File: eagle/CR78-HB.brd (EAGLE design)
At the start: 100 x 80 mm, 34 parts, among them Q1 2N3904, Q2 2N3904, Q3 2N3904, X1 22-23-2021

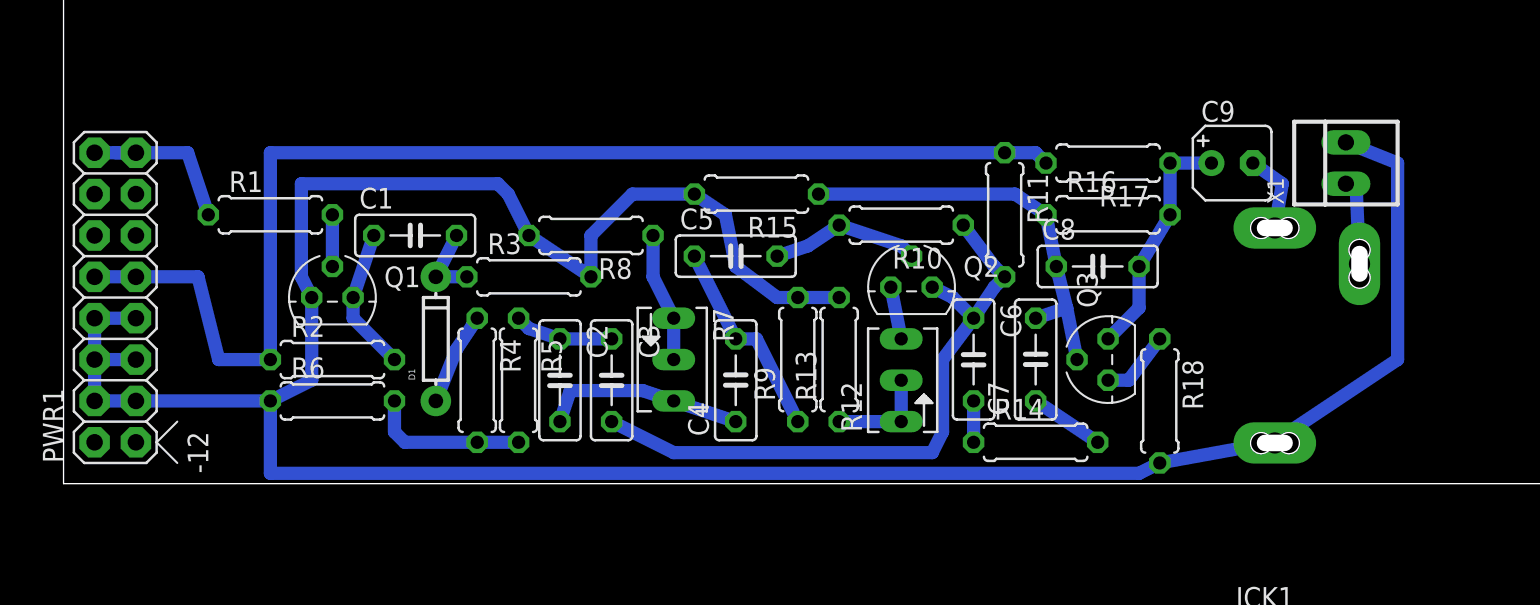
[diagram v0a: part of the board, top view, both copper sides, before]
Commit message: cutout
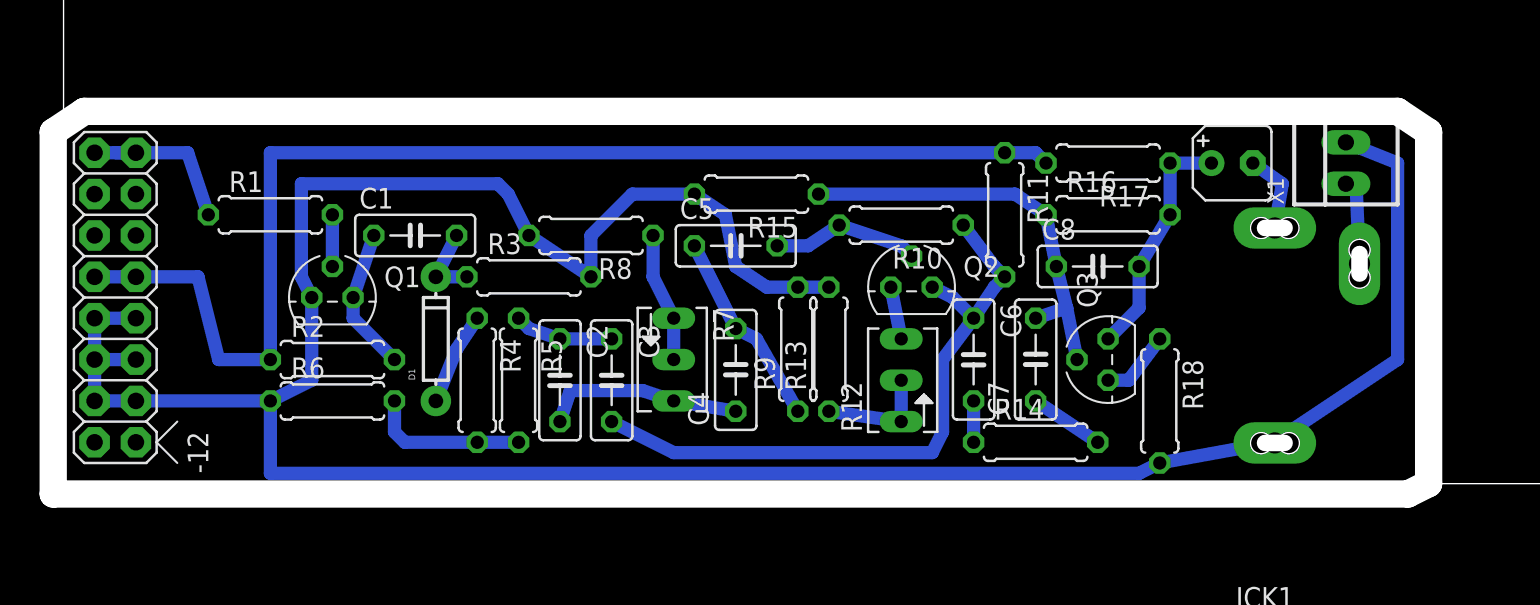
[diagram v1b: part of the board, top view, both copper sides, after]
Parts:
- moved R13 0.90 mm to (47.0, 8.26)
- moved C4 0.64 mm to (41.3, 6.99)
- moved R9 0.64 mm to (45.1, 8.26)
- moved C5 0.63 mm to (41.3, 14.6)
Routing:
- net GND: track 169.8 -> 168.9 mm
- net N$8: track 6.35 -> 7.03 mm
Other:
- board size 100 x 80 mm -> 100.6 x 80.6 mm
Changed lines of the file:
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@@
 <layer number="44" name="Drills" color="7" fill="1" visible="no" active="yes"/>
 <layer number="45" name="Holes" color="7" fill="1" visible="no" active="yes"/>
-<layer number="46" name="Milling" color="3" fill="1" visible="no" active="yes"/>
+<layer number="46" name="Milling" color="3" fill="1" visible="yes" active="yes"/>
 <layer number="47" name="Measures" color="7" fill="1" visible="no" active="yes"/>
 <layer number="48" name="Document" color="7" fill="1" visible="yes" active="yes"/>
@@
 <wire x1="100" y1="80" x2="0" y2="80" width="0" layer="20"/>
 <wire x1="0" y1="80" x2="0" y2="0" width="0" layer="20"/>
+<wire x1="-0.635" y1="-0.635" x2="-0.635" y2="21.59" width="1.6764" layer="46"/>
+<wire x1="-0.635" y1="21.59" x2="1.27" y2="22.86" width="1.6764" layer="46"/>
+<wire x1="1.27" y1="22.86" x2="81.915" y2="22.86" width="1.6764" layer="46"/>
+<wire x1="81.915" y1="22.86" x2="83.82" y2="21.59" width="1.6764" layer="46"/>
+<wire x1="83.82" y1="21.59" x2="83.82" y2="0" width="1.6764" layer="46"/>
+<wire x1="83.82" y1="0" x2="82.55" y2="-0.635" width="1.6764" layer="46"/>
+<wire x1="82.55" y1="-0.635" x2="-0.635" y2="-0.635" width="1.6764" layer="46"/>
 </plain>
 <attributes>
@@
 <element name="C2" library="rcl" package="C050-025X075" value="8n2" x="30.48" y="6.35" rot="R270"/>
 <element name="C3" library="rcl" package="C050-025X075" value="8n2" x="33.655" y="6.35" rot="R270"/>
-<element name="C4" library="rcl" package="C050-025X075" value="6n8" x="41.275" y="6.35" rot="R90"/>
-<element name="C5" library="rcl" package="C050-025X075" value="6n8" x="41.275" y="13.97"/>
+<element name="C4" library="rcl" package="C050-025X075" value="6n8" x="41.275" y="6.985" rot="R90"/>
+<element name="C5" library="rcl" package="C050-025X075" value="6n8" x="41.275" y="14.605"/>
 <element name="C6" library="rcl" package="C050-025X075" value="2n2" x="55.88" y="7.62" rot="R270"/>
 <element name="C7" library="rcl" package="C050-025X075" value="473" x="59.69" y="7.62" rot="R90"/>
@@
 <element name="R5" library="rcl" package="0207/7" value="15k" x="27.94" y="6.35" rot="R270"/>
 <element name="R8" library="rcl" package="0207/7" value="10k" x="32.385" y="15.24" rot="R180"/>
-<element name="R9" library="rcl" package="0207/7" value="15k" x="45.085" y="7.62" rot="R90"/>
-<element name="R13" library="rcl" package="0207/7" value="100R" x="47.625" y="7.62" rot="R90"/>
+<element name="R9" library="rcl" package="0207/7" value="15k" x="45.085" y="8.255" rot="R90"/>
+<element name="R13" library="rcl" package="0207/7" value="100R" x="46.99" y="8.255" rot="R90"/>
 <element name="R10" library="rcl" package="0207/7" value="1M5" x="51.435" y="15.875" rot="R180"/>
 <element name="R11" library="rcl" package="0207/7" value="10k" x="57.785" y="16.51" rot="R270"/>
@@
 <wire x1="1.905" y1="7.62" x2="1.905" y2="10.16" width="0.8128" layer="16"/>
 <wire x1="4.445" y1="5.08" x2="12.7" y2="5.08" width="0.8128" layer="16"/>
-<wire x1="47.625" y1="11.43" x2="45.085" y2="11.43" width="0.8128" layer="16"/>
+<wire x1="46.99" y1="12.065" x2="45.085" y2="12.065" width="0.8128" layer="16"/>
 <wire x1="14.605" y1="12.7" x2="15.24" y2="11.43" width="0.8128" layer="16"/>
 <wire x1="14.605" y1="18.415" x2="14.605" y2="12.7" width="0.8128" layer="16"/>
@@
 <wire x1="12.7" y1="0.635" x2="66.04" y2="0.635" width="0.8128" layer="16"/>
 <wire x1="12.7" y1="5.08" x2="12.7" y2="0.635" width="0.8128" layer="16"/>
-<wire x1="41.275" y1="13.335" x2="43.815" y2="11.43" width="0.8128" layer="16"/>
-<wire x1="43.815" y1="11.43" x2="45.085" y2="11.43" width="0.8128" layer="16"/>
+<wire x1="41.275" y1="13.335" x2="43.18" y2="12.065" width="0.8128" layer="16"/>
+<wire x1="43.18" y1="12.065" x2="45.085" y2="12.065" width="0.8128" layer="16"/>
 <wire x1="28.575" y1="15.24" x2="27.305" y2="17.78" width="0.8128" layer="16"/>
 <wire x1="27.305" y1="17.78" x2="26.67" y2="18.415" width="0.8128" layer="16"/>
@@
 <wire x1="35.56" y1="5.715" x2="31.115" y2="5.715" width="0.8128" layer="16"/>
 <wire x1="37.465" y1="5.08" x2="35.56" y2="5.715" width="0.8128" layer="16"/>
-<wire x1="37.465" y1="5.08" x2="41.275" y2="3.81" width="0.8128" layer="16"/>
+<wire x1="37.465" y1="5.08" x2="41.275" y2="4.445" width="0.8128" layer="16"/>
 </signal>
 <signal name="N$7">
@@
 <wire x1="47.625" y1="15.875" x2="51.435" y2="14.605" width="0.8128" layer="16"/>
 <wire x1="51.435" y1="14.605" x2="52.07" y2="13.97" width="0.8128" layer="16"/>
-<wire x1="43.815" y1="13.97" x2="45.72" y2="14.605" width="0.8128" layer="16"/>
+<wire x1="43.815" y1="14.605" x2="45.72" y2="14.605" width="0.8128" layer="16"/>
 <wire x1="45.72" y1="14.605" x2="47.625" y2="15.875" width="0.8128" layer="16"/>
 </signal>
@@
 <contactref element="R13" pad="1"/>
 <contactref element="R12" pad="S"/>
-<wire x1="51.435" y1="3.81" x2="47.625" y2="3.81" width="0.8128" layer="16"/>
+<wire x1="51.435" y1="3.81" x2="46.99" y2="4.445" width="0.8128" layer="16"/>
 <wire x1="51.435" y1="3.81" x2="51.435" y2="6.35" width="0.8128" layer="16"/>
 </signal>
@@
 <contactref element="C4" pad="2"/>
 <contactref element="R9" pad="1"/>
-<wire x1="38.735" y1="13.97" x2="41.275" y2="8.89" width="0.8128" layer="16"/>
-<wire x1="41.275" y1="8.89" x2="42.545" y2="8.89" width="0.8128" layer="16"/>
-<wire x1="42.545" y1="8.89" x2="45.085" y2="3.81" width="0.8128" layer="16"/>
+<wire x1="38.735" y1="14.605" x2="41.275" y2="9.525" width="0.8128" layer="16"/>
+<wire x1="41.275" y1="9.525" x2="42.545" y2="8.89" width="0.8128" layer="16"/>
+<wire x1="42.545" y1="8.89" x2="45.085" y2="4.445" width="0.8128" layer="16"/>
 </signal>
 <signal name="N$11">

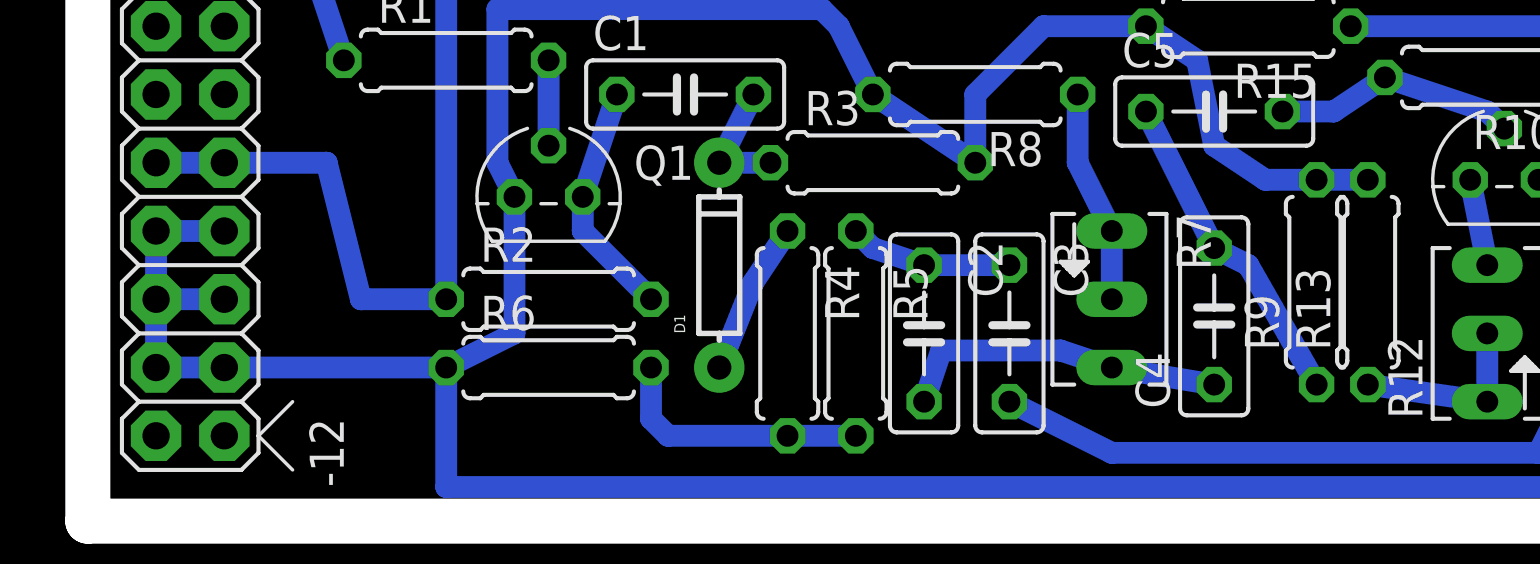
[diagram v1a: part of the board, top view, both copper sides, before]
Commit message: gcode
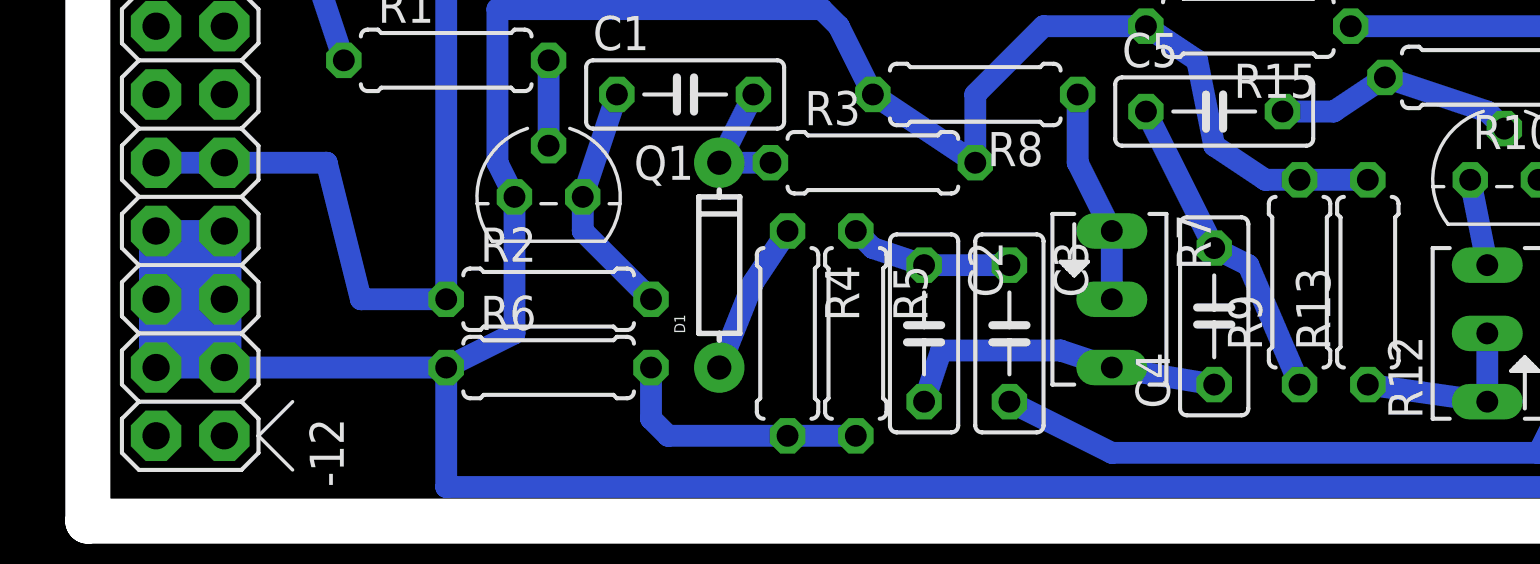
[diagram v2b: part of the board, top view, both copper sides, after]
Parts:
- moved R9 0.63 mm to (44.5, 8.26)
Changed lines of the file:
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@@
 <?xml version="1.0" encoding="utf-8"?>
 <!DOCTYPE eagle SYSTEM "eagle.dtd">
-<eagle version="7.2.0">
+<eagle version="7.1.0">
 <drawing>
 <settings>
@@
 <wire x1="83.82" y1="0" x2="82.55" y2="-0.635" width="1.6764" layer="46"/>
 <wire x1="82.55" y1="-0.635" x2="-0.635" y2="-0.635" width="1.6764" layer="46"/>
+<rectangle x1="1.27" y1="5.08" x2="5.08" y2="10.16" layer="16"/>
 </plain>
 <attributes>
@@
 <element name="R5" library="rcl" package="0207/7" value="15k" x="27.94" y="6.35" rot="R270"/>
 <element name="R8" library="rcl" package="0207/7" value="10k" x="32.385" y="15.24" rot="R180"/>
-<element name="R9" library="rcl" package="0207/7" value="15k" x="45.085" y="8.255" rot="R90"/>
+<element name="R9" library="rcl" package="0207/7" value="15k" x="44.45" y="8.255" rot="R90"/>
 <element name="R13" library="rcl" package="0207/7" value="100R" x="46.99" y="8.255" rot="R90"/>
 <element name="R10" library="rcl" package="0207/7" value="1M5" x="51.435" y="15.875" rot="R180"/>
@@
 <wire x1="1.905" y1="7.62" x2="1.905" y2="10.16" width="0.8128" layer="16"/>
 <wire x1="4.445" y1="5.08" x2="12.7" y2="5.08" width="0.8128" layer="16"/>
-<wire x1="46.99" y1="12.065" x2="45.085" y2="12.065" width="0.8128" layer="16"/>
+<wire x1="46.99" y1="12.065" x2="44.45" y2="12.065" width="0.8128" layer="16"/>
 <wire x1="14.605" y1="12.7" x2="15.24" y2="11.43" width="0.8128" layer="16"/>
 <wire x1="14.605" y1="18.415" x2="14.605" y2="12.7" width="0.8128" layer="16"/>
@@
 <wire x1="12.7" y1="5.08" x2="12.7" y2="0.635" width="0.8128" layer="16"/>
 <wire x1="41.275" y1="13.335" x2="43.18" y2="12.065" width="0.8128" layer="16"/>
-<wire x1="43.18" y1="12.065" x2="45.085" y2="12.065" width="0.8128" layer="16"/>
+<wire x1="43.18" y1="12.065" x2="44.45" y2="12.065" width="0.8128" layer="16"/>
 <wire x1="28.575" y1="15.24" x2="27.305" y2="17.78" width="0.8128" layer="16"/>
 <wire x1="27.305" y1="17.78" x2="26.67" y2="18.415" width="0.8128" layer="16"/>
@@
 <wire x1="38.735" y1="14.605" x2="41.275" y2="9.525" width="0.8128" layer="16"/>
 <wire x1="41.275" y1="9.525" x2="42.545" y2="8.89" width="0.8128" layer="16"/>
-<wire x1="42.545" y1="8.89" x2="45.085" y2="4.445" width="0.8128" layer="16"/>
+<wire x1="42.545" y1="8.89" x2="44.45" y2="4.445" width="0.8128" layer="16"/>
 </signal>
 <signal name="N$11">

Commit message: lb
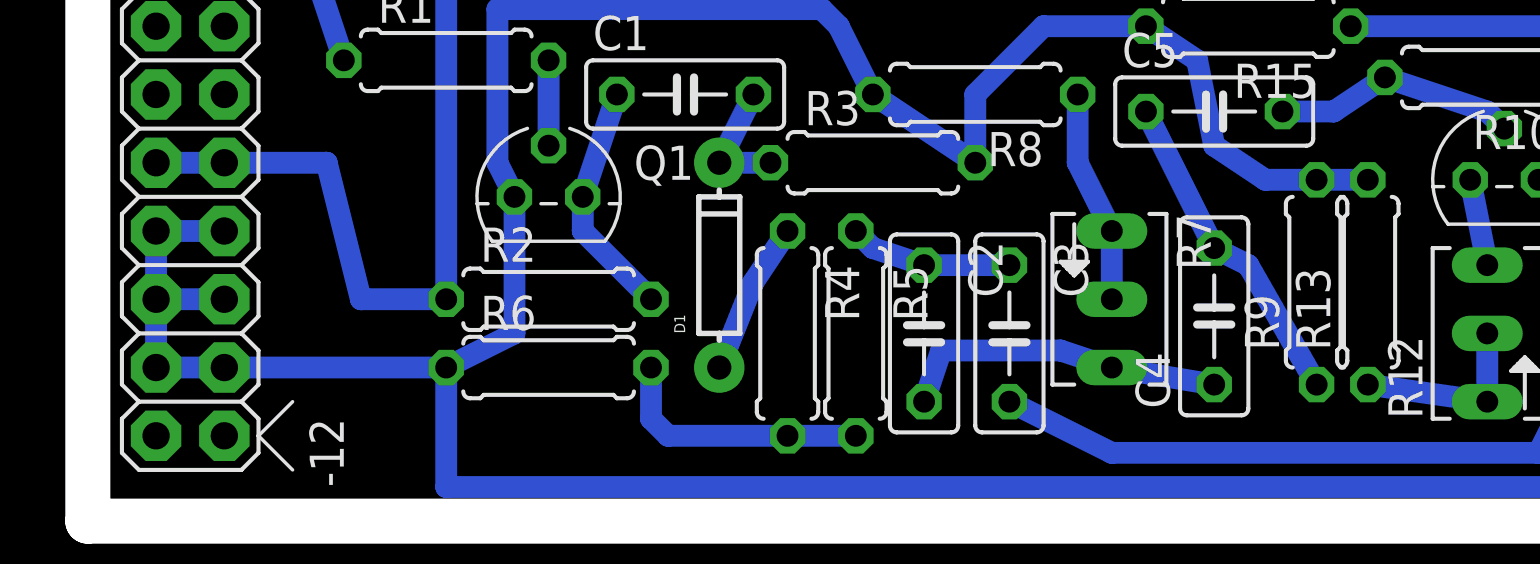
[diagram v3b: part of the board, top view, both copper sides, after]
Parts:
- C2: value 8n2 -> 12n
- C3: value 8n2 -> 18n
- C4: value 6n8 -> 12n
- C5: value 6n8 -> 10n
- C6: value 2n2 -> 8n2
- R14: value 1M5 -> 680k
- moved R9 0.63 mm to (45.1, 8.26)
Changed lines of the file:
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@@
 <?xml version="1.0" encoding="utf-8"?>
 <!DOCTYPE eagle SYSTEM "eagle.dtd">
-<eagle version="7.1.0">
+<eagle version="7.2.0">
 <drawing>
 <settings>
@@
 <wire x1="83.82" y1="0" x2="82.55" y2="-0.635" width="1.6764" layer="46"/>
 <wire x1="82.55" y1="-0.635" x2="-0.635" y2="-0.635" width="1.6764" layer="46"/>
-<rectangle x1="1.27" y1="5.08" x2="5.08" y2="10.16" layer="16"/>
 </plain>
 <attributes>
@@
 <elements>
 <element name="C1" library="rcl" package="C050-025X075" value="27n" x="21.59" y="15.24"/>
-<element name="C2" library="rcl" package="C050-025X075" value="8n2" x="30.48" y="6.35" rot="R270"/>
-<element name="C3" library="rcl" package="C050-025X075" value="8n2" x="33.655" y="6.35" rot="R270"/>
-<element name="C4" library="rcl" package="C050-025X075" value="6n8" x="41.275" y="6.985" rot="R90"/>
-<element name="C5" library="rcl" package="C050-025X075" value="6n8" x="41.275" y="14.605"/>
-<element name="C6" library="rcl" package="C050-025X075" value="2n2" x="55.88" y="7.62" rot="R270"/>
+<element name="C2" library="rcl" package="C050-025X075" value="12n" x="30.48" y="6.35" rot="R270"/>
+<element name="C3" library="rcl" package="C050-025X075" value="18n" x="33.655" y="6.35" rot="R270"/>
+<element name="C4" library="rcl" package="C050-025X075" value="12n" x="41.275" y="6.985" rot="R90"/>
+<element name="C5" library="rcl" package="C050-025X075" value="10n" x="41.275" y="14.605"/>
+<element name="C6" library="rcl" package="C050-025X075" value="8n2" x="55.88" y="7.62" rot="R270"/>
 <element name="C7" library="rcl" package="C050-025X075" value="473" x="59.69" y="7.62" rot="R90"/>
 <element name="C8" library="rcl" package="C050-025X075" value="47p" x="63.5" y="13.335"/>
@@
 <element name="Q3" library="808_lt" package="TO92" value="2N3904" x="64.135" y="7.62" rot="R90"/>
 <element name="R3" library="rcl" package="0207/7" value="270k" x="28.575" y="12.7"/>
-<element name="R14" library="rcl" package="0207/7" value="1M5" x="59.69" y="2.54"/>
+<element name="R14" library="rcl" package="0207/7" value="680k" x="59.69" y="2.54"/>
 <element name="R16" library="rcl" package="0207/7" value="470k" x="64.135" y="16.51"/>
 <element name="R17" library="rcl" package="0207/7" value="47k" x="64.135" y="19.685" rot="R180"/>
@@
 <element name="R5" library="rcl" package="0207/7" value="15k" x="27.94" y="6.35" rot="R270"/>
 <element name="R8" library="rcl" package="0207/7" value="10k" x="32.385" y="15.24" rot="R180"/>
-<element name="R9" library="rcl" package="0207/7" value="15k" x="44.45" y="8.255" rot="R90"/>
+<element name="R9" library="rcl" package="0207/7" value="15k" x="45.085" y="8.255" rot="R90"/>
 <element name="R13" library="rcl" package="0207/7" value="100R" x="46.99" y="8.255" rot="R90"/>
 <element name="R10" library="rcl" package="0207/7" value="1M5" x="51.435" y="15.875" rot="R180"/>
@@
 <wire x1="1.905" y1="7.62" x2="1.905" y2="10.16" width="0.8128" layer="16"/>
 <wire x1="4.445" y1="5.08" x2="12.7" y2="5.08" width="0.8128" layer="16"/>
-<wire x1="46.99" y1="12.065" x2="44.45" y2="12.065" width="0.8128" layer="16"/>
+<wire x1="46.99" y1="12.065" x2="45.085" y2="12.065" width="0.8128" layer="16"/>
 <wire x1="14.605" y1="12.7" x2="15.24" y2="11.43" width="0.8128" layer="16"/>
 <wire x1="14.605" y1="18.415" x2="14.605" y2="12.7" width="0.8128" layer="16"/>
@@
 <wire x1="12.7" y1="5.08" x2="12.7" y2="0.635" width="0.8128" layer="16"/>
 <wire x1="41.275" y1="13.335" x2="43.18" y2="12.065" width="0.8128" layer="16"/>
-<wire x1="43.18" y1="12.065" x2="44.45" y2="12.065" width="0.8128" layer="16"/>
+<wire x1="43.18" y1="12.065" x2="45.085" y2="12.065" width="0.8128" layer="16"/>
 <wire x1="28.575" y1="15.24" x2="27.305" y2="17.78" width="0.8128" layer="16"/>
 <wire x1="27.305" y1="17.78" x2="26.67" y2="18.415" width="0.8128" layer="16"/>
@@
 <wire x1="38.735" y1="14.605" x2="41.275" y2="9.525" width="0.8128" layer="16"/>
 <wire x1="41.275" y1="9.525" x2="42.545" y2="8.89" width="0.8128" layer="16"/>
-<wire x1="42.545" y1="8.89" x2="44.45" y2="4.445" width="0.8128" layer="16"/>
+<wire x1="42.545" y1="8.89" x2="45.085" y2="4.445" width="0.8128" layer="16"/>
 </signal>
 <signal name="N$11">
